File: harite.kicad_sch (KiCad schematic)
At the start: 38 parts, among them J1 Cirque Connector, U1 RP2040_Zero

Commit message: Use skrhade switch model
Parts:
- S1, S2, S3, S4, S5: footprint footprints:SKRHADE010 -> footprints:SKRHADE
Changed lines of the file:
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@@
 			)
 		)
-		(property "Footprint" "footprints:SKRHADE010"
+		(property "Footprint" "footprints:SKRHADE"
 			(at 59.69 143.18 0)
 			(effects
@@
 			)
 		)
-		(property "Footprint" "footprints:SKRHADE010"
+		(property "Footprint" "footprints:SKRHADE"
 			(at 129.54 143.18 0)
 			(effects
@@
 			)
 		)
-		(property "Footprint" "footprints:SKRHADE010"
+		(property "Footprint" "footprints:SKRHADE"
 			(at 267.97 206.68 0)
 			(effects
@@
 			)
 		)
-		(property "Footprint" "footprints:SKRHADE010"
+		(property "Footprint" "footprints:SKRHADE"
 			(at 199.39 143.18 0)
 			(effects
@@
 			)
 		)
-		(property "Footprint" "footprints:SKRHADE010"
+		(property "Footprint" "footprints:SKRHADE"
 			(at 269.24 143.18 0)
 			(effects

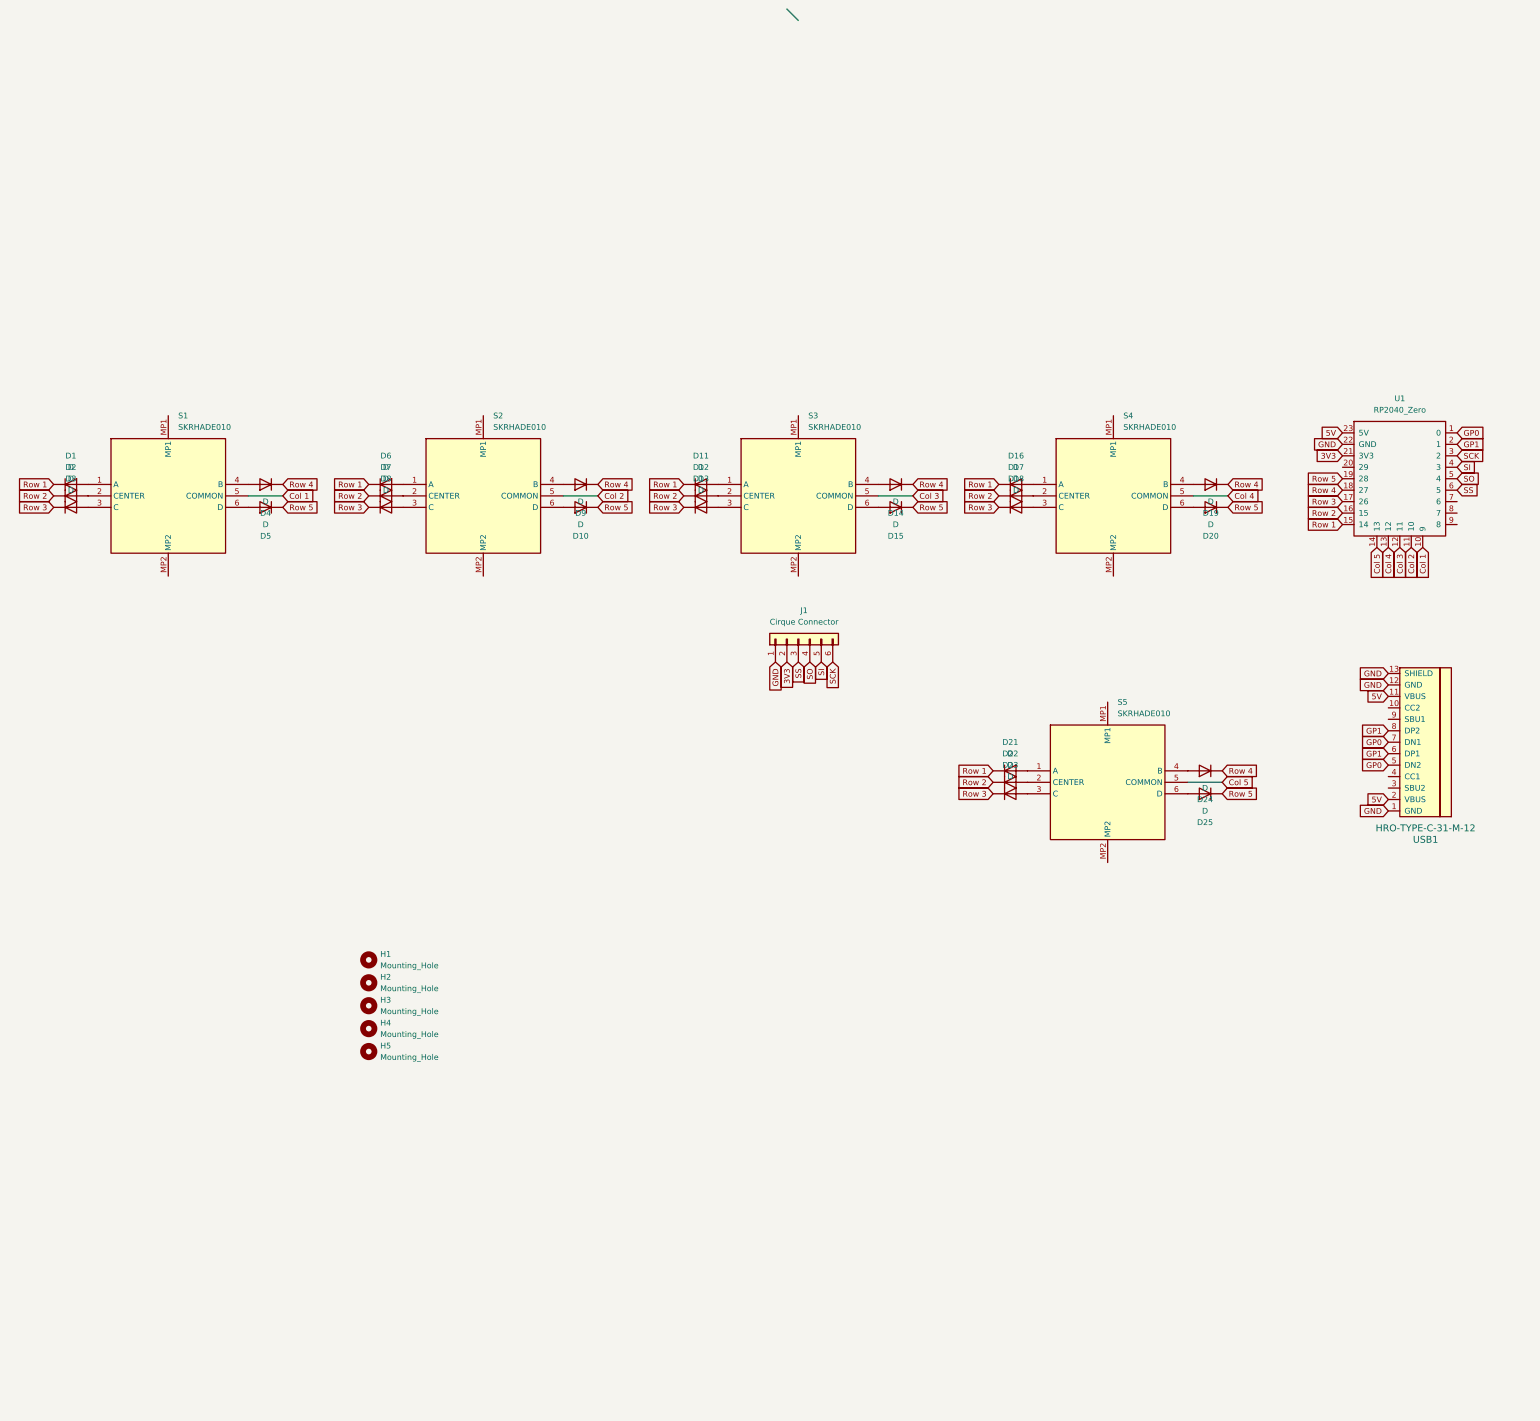
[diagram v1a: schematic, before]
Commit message: Mirror sides
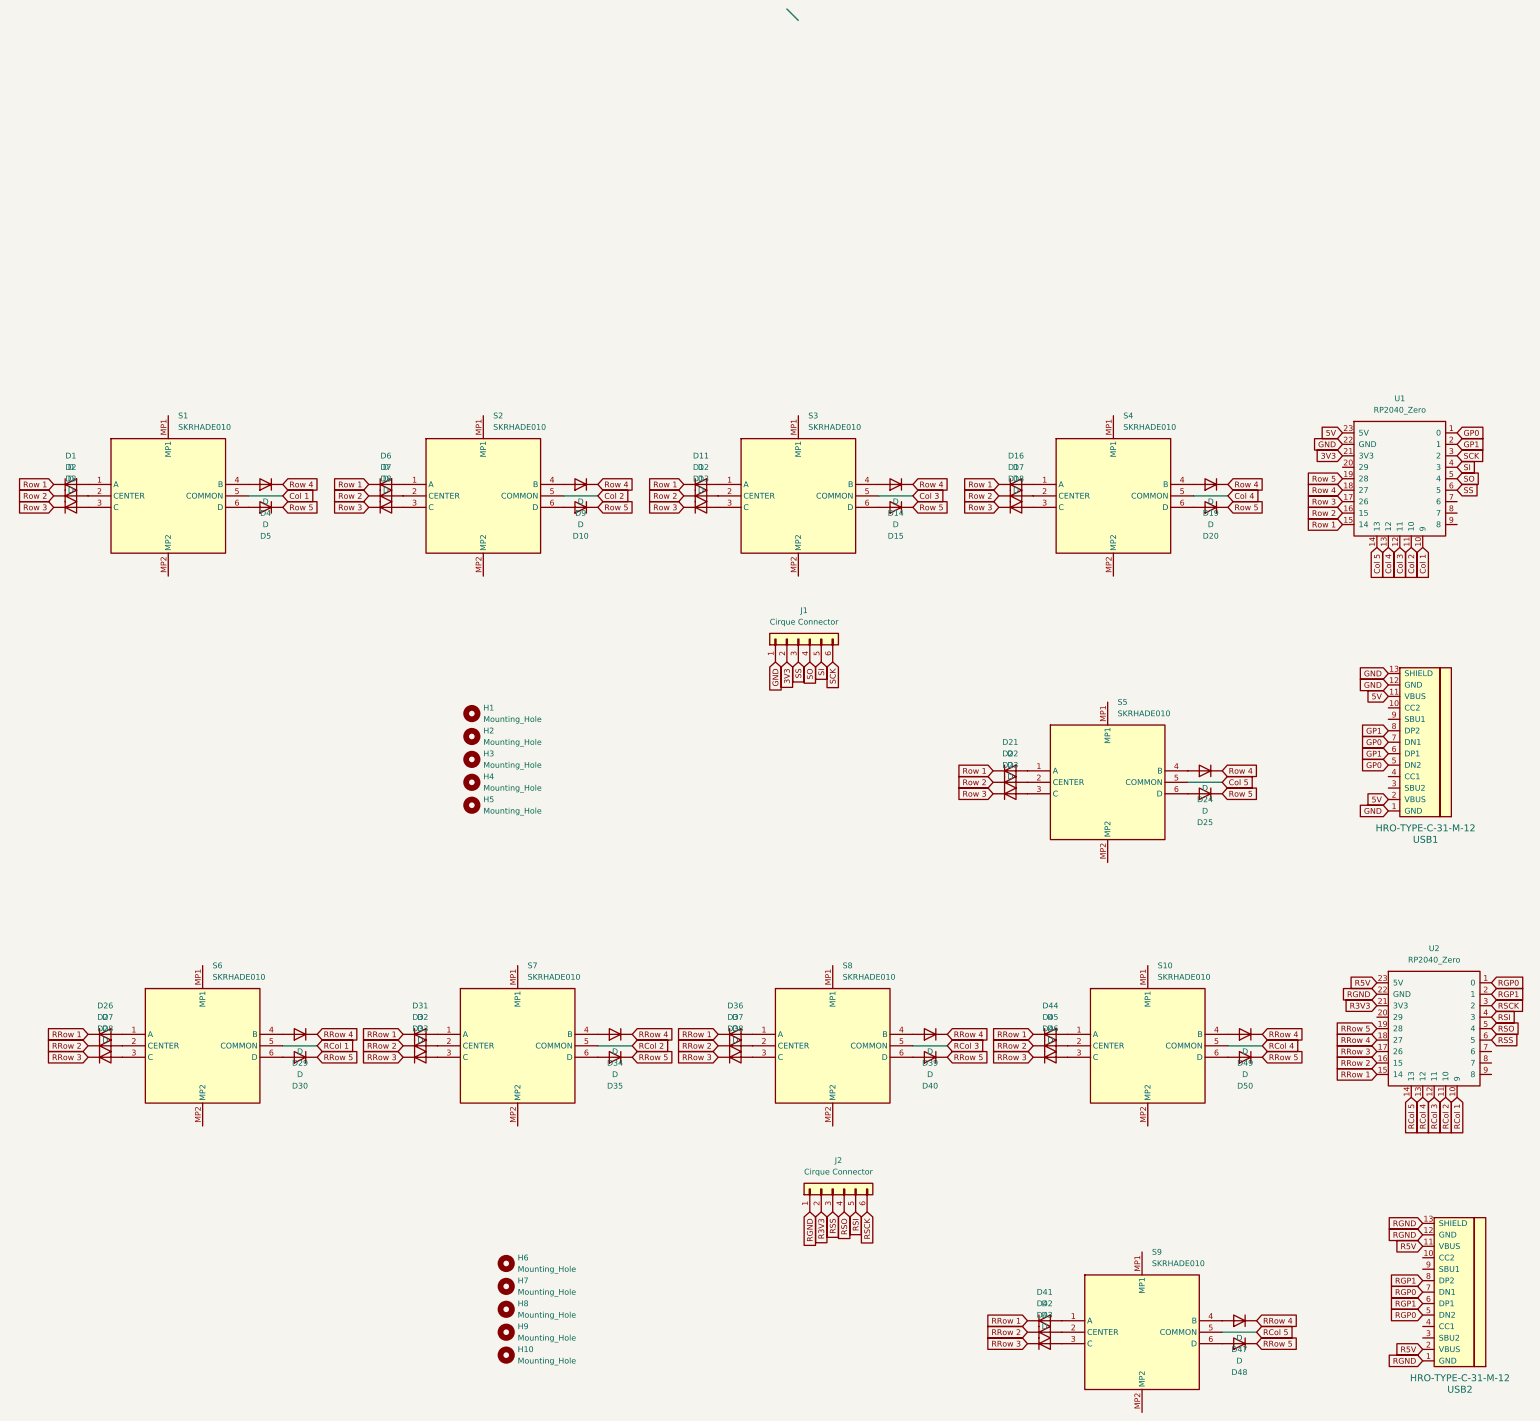
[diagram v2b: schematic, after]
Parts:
- added D26, D27, D28, D29, D30, D31, D32, D33, D34, D35, D36, D37, D38, D39, D40, D41, D42, D43, D44, D45, D46, D47, D48, D49, D50: D, ScottoKeebs_Components:Diode_SOD-123, symbol Device:D
- added H10, H6, H7, H8, H9: Mounting_Hole, MountingHole:MountingHole_2.2mm_M2_Pad_Via, symbol ScottoKeebs:Placeholder_Mounting_Hole
- added J2: Cirque Connector, footprints:Cirque-connector, symbol Connector_Generic:Conn_01x06
- added S10, S6, S7, S8, S9: SKRHADE010, footprints:SKRHADE, symbol SKRHADE010:SKRHADE010
- added U2: RP2040_Zero, ScottoKeebs_MCU:RP2040_Zero, symbol ScottoKeebs:MCU_RP2040_Zero
- added USB2: HRO-TYPE-C-31-M-12, footprints:HRO-TYPE-C-31-M-12, symbol USBType-C:HRO-TYPE-C-31-M-12
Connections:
- new net: D36.2 (A), S8.1 (A)
- new net: D37.2 (A), S8.2 (CENTER)
- new net: D38.2 (A), S8.3 (C)
- new net: D39.2 (A), S8.4 (B)
- new net: D40.2 (A), S8.6 (D)
- new net: D35.2 (A), S7.6 (D)
- new net: D45.2 (A), S10.2 (CENTER)
- new net: D44.2 (A), S10.1 (A)
- new net: D46.2 (A), S10.3 (C)
- new net: D49.2 (A), S10.4 (B)
- new net: D50.2 (A), S10.6 (D)
- new net: D41.2 (A), S9.1 (A)
- new net: D31.2 (A), S7.1 (A)
- new net: D43.2 (A), S9.3 (C)
- new net: D27.2 (A), S6.2 (CENTER)
- new net: D42.2 (A), S9.2 (CENTER)
- new net: D30.2 (A), S6.6 (D)
- new net: D34.2 (A), S7.4 (B)
- new net: D47.2 (A), S9.4 (B)
- new net: D32.2 (A), S7.2 (CENTER)
- new net: D33.2 (A), S7.3 (C)
- new net: D26.2 (A), S6.1 (A)
- new net: D48.2 (A), S9.6 (D)
- new net: D28.2 (A), S6.3 (C)
- new net: D29.2 (A), S6.4 (B)
- new net R3V3: J2.2 (Pin_2), U2.21 (3V3)
- new net R5V: U2.23 (5V), USB2.11 (VBUS), USB2.2 (VBUS)
- new net RCol 1: S6.5 (COMMON), U2.10 (9)
- new net RCol 2: S7.5 (COMMON), U2.11 (10)
- new net RCol 3: S8.5 (COMMON), U2.12 (11)
- new net RCol 4: S10.5 (COMMON), U2.13 (12)
- new net RCol 5: S9.5 (COMMON), U2.14 (13)
- new net RGND: J2.1 (Pin_1), U2.22 (GND), USB2.1 (GND), USB2.12 (GND), USB2.13 (SHIELD)
- new net RGP0: U2.1 (0), USB2.5 (DN2), USB2.7 (DN1)
- new net RGP1: U2.2 (1), USB2.6 (DP1), USB2.8 (DP2)
- new net RRow 1: D26.1 (K), D31.1 (K), D36.1 (K), D41.1 (K), D44.1 (K), U2.15 (14)
- new net RRow 2: D27.1 (K), D32.1 (K), D37.1 (K), D42.1 (K), D45.1 (K), U2.16 (15)
- new net RRow 3: D28.1 (K), D33.1 (K), D38.1 (K), D43.1 (K), D46.1 (K), U2.17 (26)
- new net RRow 4: D29.1 (K), D34.1 (K), D39.1 (K), D47.1 (K), D49.1 (K), U2.18 (27)
- new net RRow 5: D30.1 (K), D35.1 (K), D40.1 (K), D48.1 (K), D50.1 (K), U2.19 (28)
- new net RSCK: J2.6 (Pin_6), U2.3 (2)
- new net RSI: J2.5 (Pin_5), U2.4 (3)
- new net RSO: J2.4 (Pin_4), U2.5 (4)
- new net RSS: J2.3 (Pin_3), U2.6 (5)
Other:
- moved on the sheet: H1, H2, H3, H4, H5
